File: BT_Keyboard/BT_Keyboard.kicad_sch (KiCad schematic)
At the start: 163 parts, among them J1 Conn_01x22_Pin, J2 Conn_01x22_Pin, J3 Conn_01x14_Pin, J4 Conn_01x22_Pin, J5 Conn_01x22_Pin, J7 Speaker, J8 Battery 5V, SW1 SW_Push_45deg, SW10 SW_Push_45deg, SW11 SW_Push_45deg, SW12 SW_Push_45deg, SW13 SW_Push_45deg, SW14 SW_Push_45deg, SW15 SW_Push_45deg, SW16 SW_Push_45deg, SW17 SW_Push_45deg, SW18 SW_Push_45deg, SW19 SW_Push_45deg, SW2 SW_Push_45deg, SW20 SW_Push_45deg, SW21 SW_Push_45deg, SW22 SW_Push_45deg, SW23 SW_Push_45deg, SW24 SW_Push_45deg, SW25 SW_Push_45deg, SW26 SW_Push_45deg, SW27 SW_Push_45deg, SW28 Backspace, SW29 Tab, SW3 SW_Push_45deg, SW30 SW_Push_45deg, SW31 SW_Push_45deg, SW32 SW_Push_45deg, SW33 SW_Push_45deg, SW34 SW_Push_45deg, SW35 SW_Push_45deg, SW36 SW_Push_45deg, SW37 SW_Push_45deg, SW38 SW_Push_45deg, SW39 SW_Push_45deg, SW4 SW_Push_45deg, SW40 SW_Push_45deg, SW41 SW_Push_45deg, SW42 SW_Push_45deg, SW43 Cap, SW44 SW_Push_45deg, SW45 SW_Push_45deg, SW46 SW_Push_45deg, SW47 SW_Push_45deg, SW48 SW_Push_45deg, SW49 SW_Push_45deg, SW5 SW_Push_45deg, SW50 SW_Push_45deg, SW51 SW_Push_45deg, SW52 SW_Push_45deg, SW53 SW_Push_45deg, SW54 SW_Push_45deg, SW55 Enter, SW56 Shift, SW57 SW_Push_45deg, SW58 SW_Push_45deg, SW59 SW_Push_45deg, SW6 SW_Push_45deg, SW60 SW_Push_45deg, SW61 SW_Push_45deg, SW62 SW_Push_45deg, SW63 SW_Push_45deg, SW64 SW_Push_45deg, SW65 SW_Push_45deg, SW66 SW_Push_45deg, SW67 SW_Push_45deg, SW68 SW_Push_45deg, SW69 SW_Push_45deg, SW7 SW_Push_45deg, SW70 SW_Push_45deg, SW71 SW_Push_45deg, SW72 SW_Push_45deg, SW73 SW_Push_45deg, SW74 SW_Push_45deg, SW75 SW_Push_45deg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

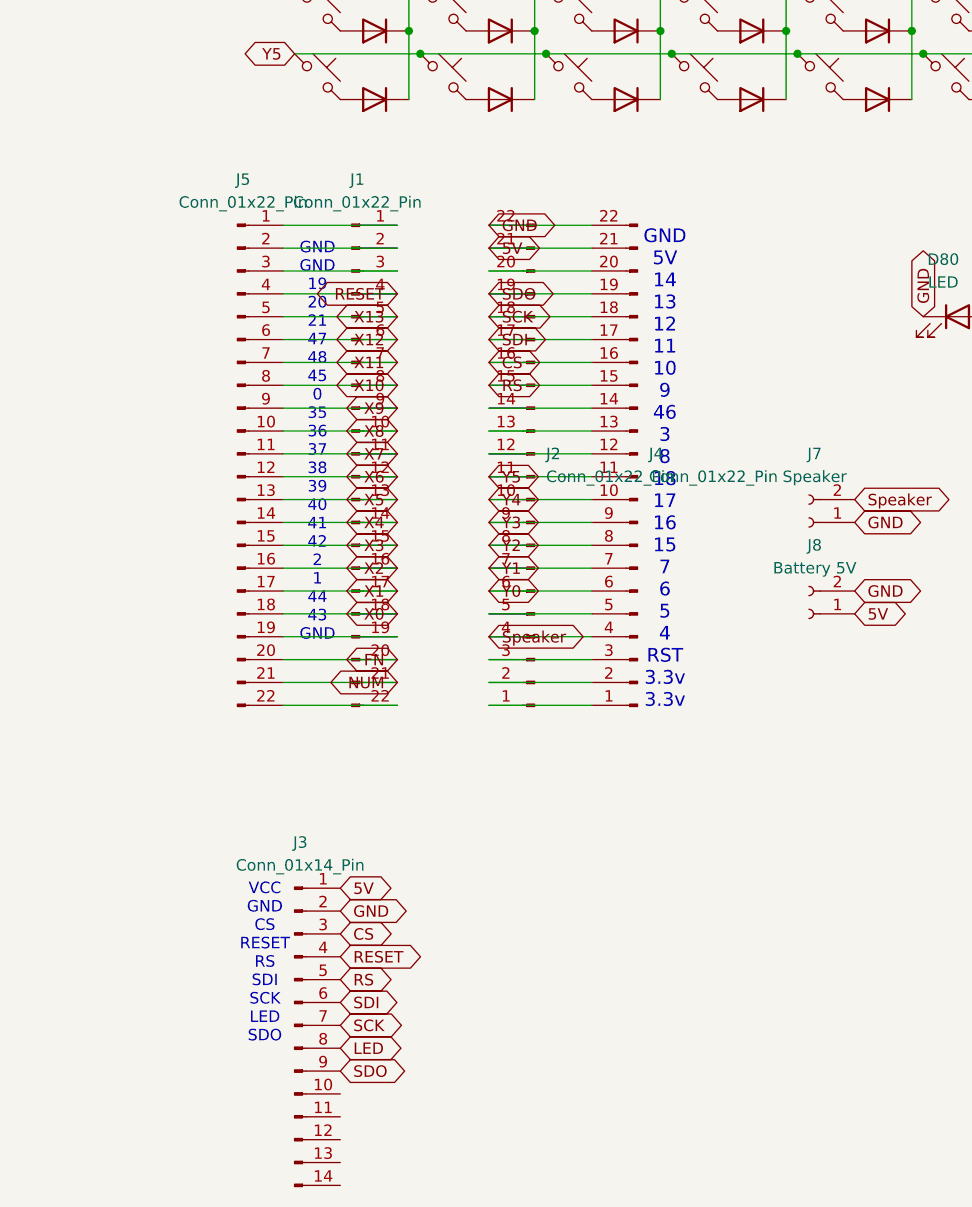
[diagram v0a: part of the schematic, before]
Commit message: Add files via upload
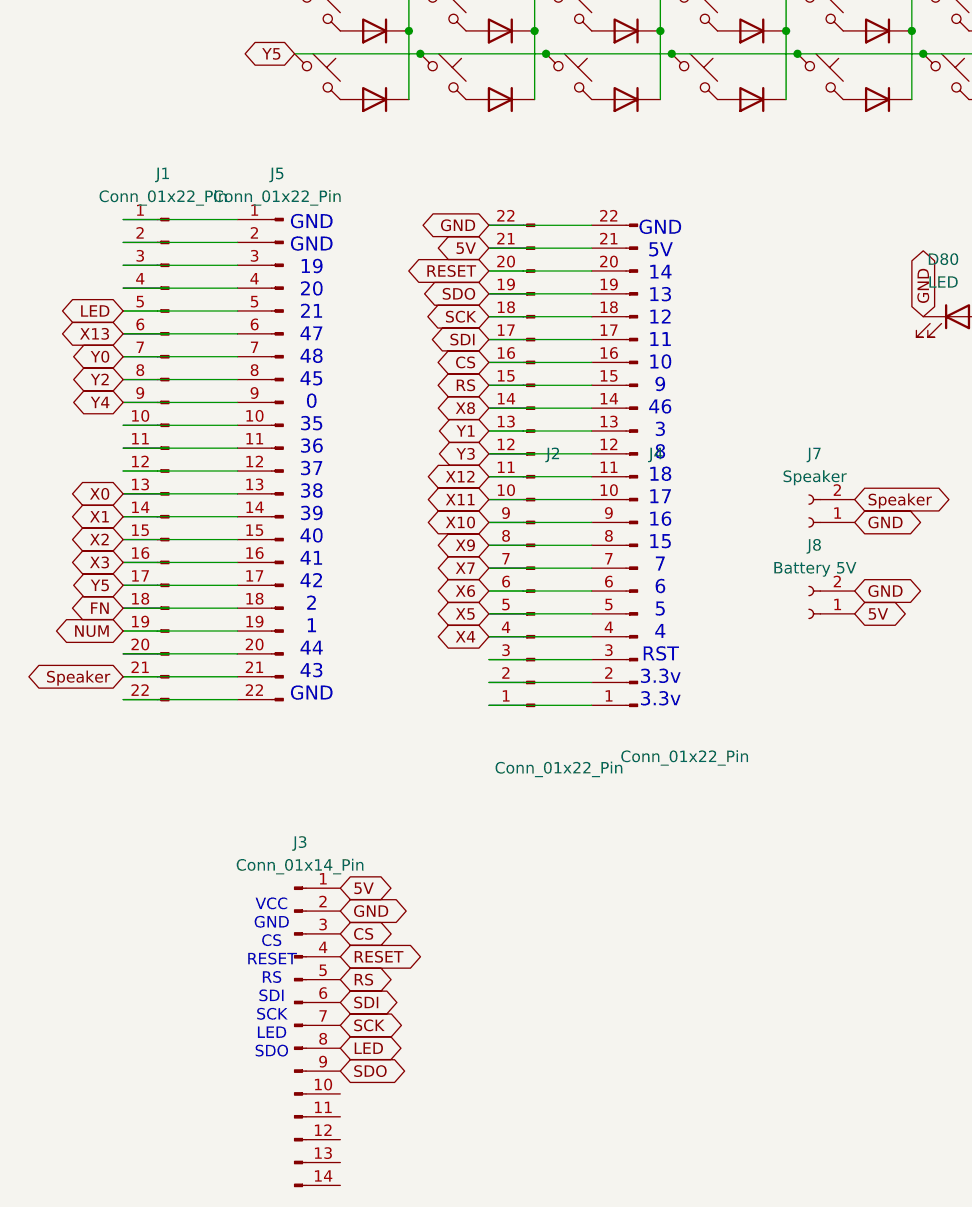
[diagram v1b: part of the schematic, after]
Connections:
- net FN: now also J1.18 (Pin_18), J5.18 (Pin_18); no longer J1.20 (Pin_20), J5.20 (Pin_20)
- net LED: now also J1.5 (Pin_5), J5.5 (Pin_5)
- net NUM: now also J1.19 (Pin_19), J5.19 (Pin_19); no longer J1.21 (Pin_21), J5.21 (Pin_21)
- net RESET: now also J2.20 (Pin_20), J4.20 (Pin_20); no longer J1.4 (Pin_4), J5.4 (Pin_4)
- net Speaker: now also J1.21 (Pin_21), J5.21 (Pin_21); no longer J2.4 (Pin_4), J4.4 (Pin_4)
- net X0: now also J1.13 (Pin_13), J5.13 (Pin_13); no longer J1.18 (Pin_18), J5.18 (Pin_18)
- net X1: now also J1.14 (Pin_14), J5.14 (Pin_14); no longer J1.17 (Pin_17), J5.17 (Pin_17)
- net X10: now also J2.9 (Pin_9), J4.9 (Pin_9); no longer J1.8 (Pin_8), J5.8 (Pin_8)
- net X11: now also J2.10 (Pin_10), J4.10 (Pin_10); no longer J1.7 (Pin_7), J5.7 (Pin_7)
- net X12: now also J2.11 (Pin_11), J4.11 (Pin_11); no longer J1.6 (Pin_6), J5.6 (Pin_6)
- net X13: now also J1.6 (Pin_6), J5.6 (Pin_6); no longer J1.5 (Pin_5), J5.5 (Pin_5)
- net X2: now also J1.15 (Pin_15), J5.15 (Pin_15); no longer J1.16 (Pin_16), J5.16 (Pin_16)
- net X3: now also J1.16 (Pin_16), J5.16 (Pin_16); no longer J1.15 (Pin_15), J5.15 (Pin_15)
- net X4: now also J2.4 (Pin_4), J4.4 (Pin_4); no longer J1.14 (Pin_14), J5.14 (Pin_14)
- net X5: now also J2.5 (Pin_5), J4.5 (Pin_5); no longer J1.13 (Pin_13), J5.13 (Pin_13)
- net X6: now also J2.6 (Pin_6), J4.6 (Pin_6); no longer J1.12 (Pin_12), J5.12 (Pin_12)
- net X7: now also J2.7 (Pin_7), J4.7 (Pin_7); no longer J1.11 (Pin_11), J5.11 (Pin_11)
- net X8: now also J2.14 (Pin_14), J4.14 (Pin_14); no longer J1.10 (Pin_10), J5.10 (Pin_10)
- net X9: now also J2.8 (Pin_8), J4.8 (Pin_8); no longer J1.9 (Pin_9), J5.9 (Pin_9)
- net Y0: now also J1.7 (Pin_7), J5.7 (Pin_7); no longer J2.6 (Pin_6), J4.6 (Pin_6)
- net Y1: now also J2.13 (Pin_13), J4.13 (Pin_13); no longer J2.7 (Pin_7), J4.7 (Pin_7)
- net Y2: now also J1.8 (Pin_8), J5.8 (Pin_8); no longer J2.8 (Pin_8), J4.8 (Pin_8)
- net Y3: now also J2.12 (Pin_12), J4.12 (Pin_12); no longer J2.9 (Pin_9), J4.9 (Pin_9)
- net Y4: now also J1.9 (Pin_9), J5.9 (Pin_9); no longer J2.10 (Pin_10), J4.10 (Pin_10)
- net Y5: now also J1.17 (Pin_17), J5.17 (Pin_17); no longer J2.11 (Pin_11), J4.11 (Pin_11)
- new net: J1.10 (Pin_10), J5.10 (Pin_10)
- new net: J1.11 (Pin_11), J5.11 (Pin_11)
- new net: J1.12 (Pin_12), J5.12 (Pin_12)
- new net: J1.20 (Pin_20), J5.20 (Pin_20)
- new net: J1.4 (Pin_4), J5.4 (Pin_4)
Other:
- moved on the sheet: J1, J5
